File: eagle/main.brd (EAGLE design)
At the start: 100 x 80 mm, 32 parts, among them Q1 BSS97, U1 LTC3789EGNPBF

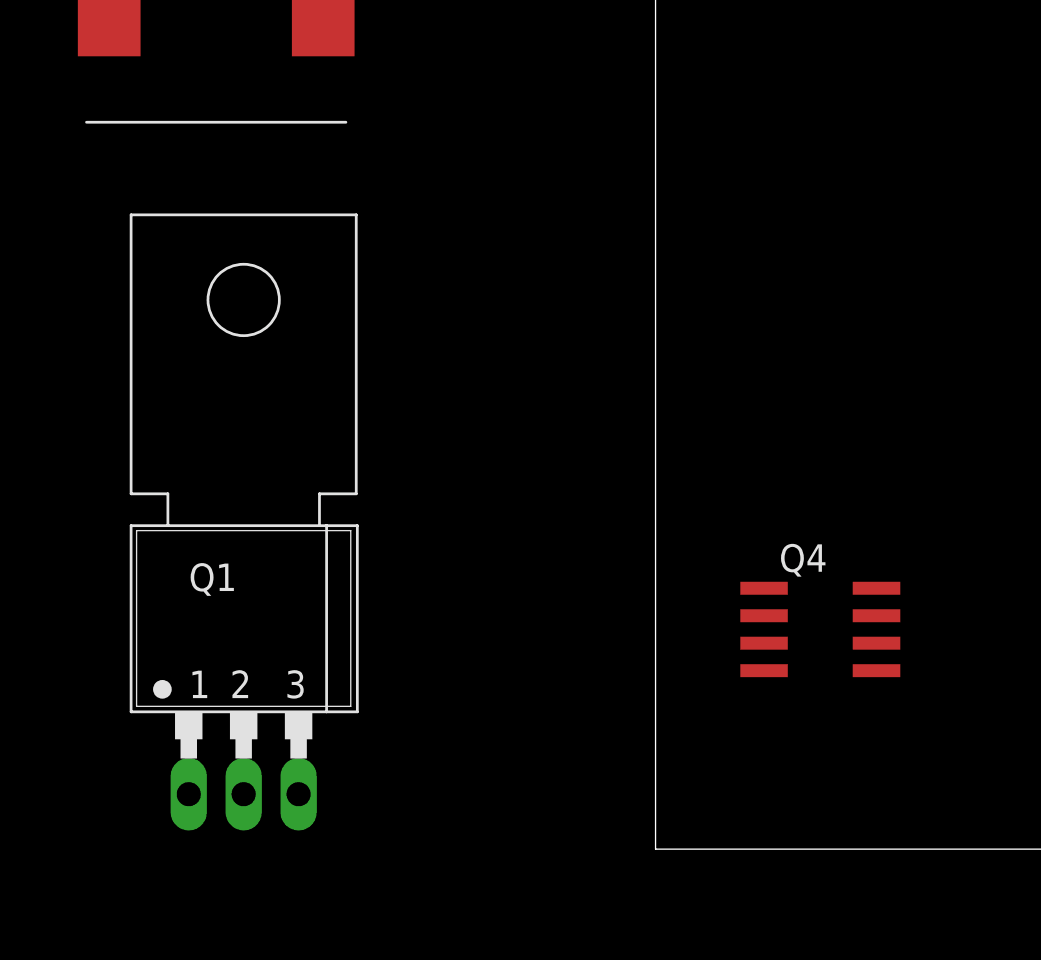
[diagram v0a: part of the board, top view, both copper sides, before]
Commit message: [ update ] sch
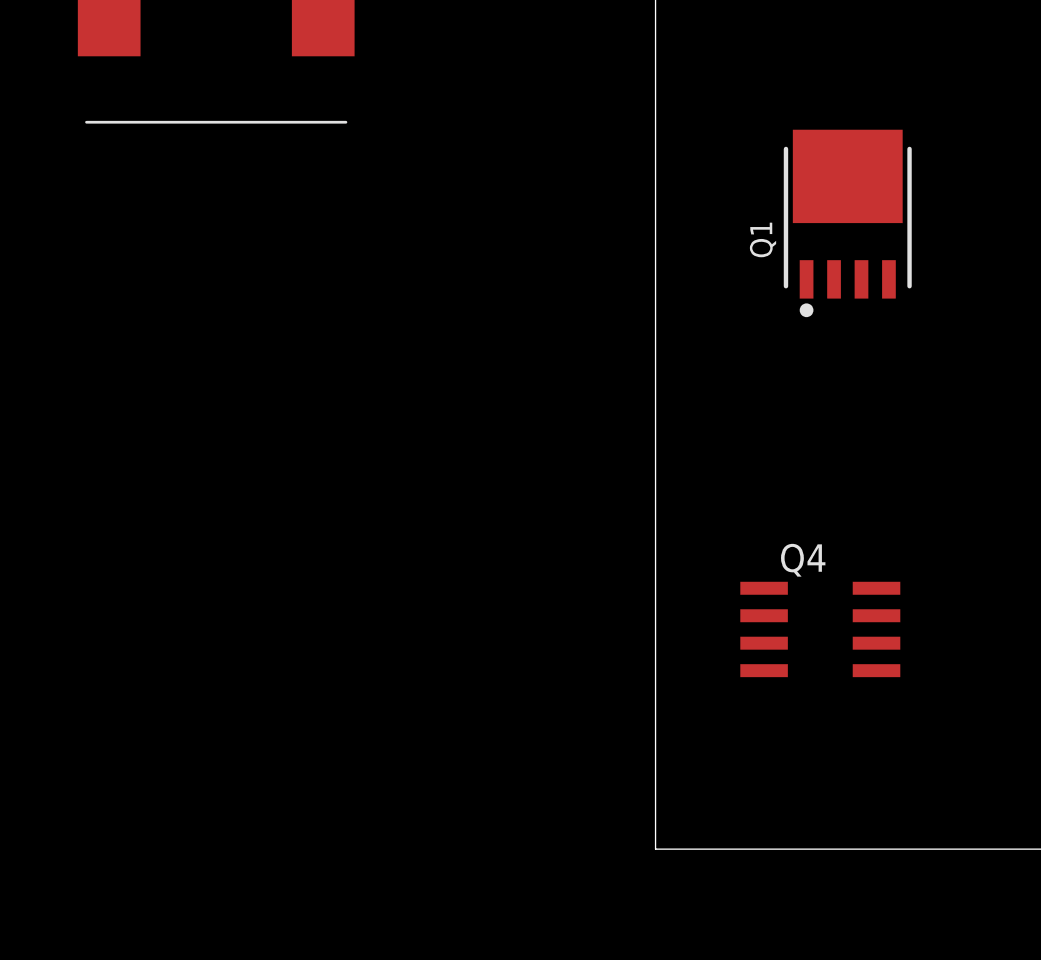
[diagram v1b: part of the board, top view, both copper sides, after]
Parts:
- Q1: value BSS97 -> SQJ886EP; device transistor-fet:TO202 -> transistor-fet:POWERPAK-SO-08
- moved Q1 35.3 mm to (8.89, 29.2)
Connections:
- net SW1: now also Q1.2, Q1.3
- net TG1: now also Q1.4; no longer Q1.3
- net VIN: now also Q1.5-8; no longer Q1.2
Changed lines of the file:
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@@
 <setting verticaltext="up"/>
 </settings>
-<grid distance="0.05" unitdist="inch" unit="inch" style="lines" multiple="1" display="no" altdistance="0.025" altunitdist="inch" altunit="inch"/>
+<grid distance="0.05" unitdist="inch" unit="inch" style="lines" multiple="1" display="yes" altdistance="0.025" altunitdist="inch" altunit="inch"/>
 <layers>
 <layer number="1" name="Top" color="4" fill="1" visible="yes" active="yes"/>
@@
 <element name="C4" library="rcl" package="C1206K" value="1u" x="-35.56" y="71.12"/>
 <element name="C5" library="rcl" package="C1206K" value="4.7u" x="-40.64" y="71.12"/>
-<element name="Q1" library="transistor-fet" package="TO202" value="BSS97" x="-19.05" y="7.62"/>
 <element name="C6" library="rcl" package="C1206K" value="2.2u" x="-45.72" y="71.12"/>
 <element name="C7" library="rcl" package="PANASONIC_A" value="330u" x="-66.04" y="33.02"/>
@@
 <element name="Q3" library="transistor-power" package="SO-08" value="" x="-91.44" y="-21.59"/>
 <element name="Q4" library="transistor-power" package="SO-08" value="" x="7.62" y="10.16" rot="R270"/>
+<element name="Q1" library="transistor-fet" package="POWERPAK-SO-08" value="SQJ886EP" x="8.89" y="29.21"/>
 </elements>
 <signals>
@@
 <contactref element="R10" pad="1"/>
 <contactref element="C8" pad="1"/>
-<contactref element="Q1" pad="2"/>
-<wire x1="-56.032" y1="64.77" x2="-52.3" y2="71.12" width="0" layer="19" extent="1-1"/>
-<wire x1="-51.9938" y1="36.5252" x2="-56.032" y2="64.77" width="0" layer="19" extent="1-1"/>
-<wire x1="-19.05" y1="2.54" x2="-51.9938" y2="36.5252" width="0" layer="19" extent="1-1"/>
+<contactref element="Q1" pad="5-8"/>
+<wire x1="-51.9938" y1="36.5252" x2="8.89" y2="31.115" width="0" layer="19" extent="1-1"/>
+<wire x1="-56.032" y1="64.77" x2="-51.9938" y2="36.5252" width="0" layer="19" extent="1-1"/>
+<wire x1="-52.3" y1="71.12" x2="-56.032" y2="64.77" width="0" layer="19" extent="1-1"/>
 </signal>
 <signal name="SENSE-">
@@
 <signal name="TG1">
 <contactref element="U1" pad="26"/>
-<contactref element="Q1" pad="3"/>
-<wire x1="-47.0662" y1="40.9448" x2="-16.51" y2="2.54" width="0" layer="19" extent="1-1"/>
+<contactref element="Q1" pad="4"/>
+<wire x1="-47.0662" y1="40.9448" x2="10.795" y2="26.3525" width="0" layer="19" extent="1-1"/>
 </signal>
 <signal name="BG2">
@@
 <signal name="SW1">
 <contactref element="U1" pad="27"/>
-<contactref element="Q1" pad="1"/>
 <contactref element="L1" pad="2"/>
 <contactref element="C12" pad="1"/>
@@
 <contactref element="Q2" pad="6"/>
 <contactref element="Q2" pad="7"/>
+<contactref element="Q1" pad="1"/>
+<contactref element="Q1" pad="2"/>
+<contactref element="Q1" pad="3"/>
+<wire x1="8.255" y1="26.3525" x2="6.985" y2="26.3525" width="0" layer="19" extent="1-1"/>
+<wire x1="9.525" y1="26.3525" x2="8.255" y2="26.3525" width="0" layer="19" extent="1-1"/>
+<wire x1="-84.455" y1="-18.99" x2="9.525" y2="26.3525" width="0" layer="19" extent="1-1"/>
 <wire x1="-83.185" y1="-18.99" x2="-84.455" y2="-18.99" width="0" layer="19" extent="1-1"/>
 <wire x1="-81.915" y1="-18.99" x2="-83.185" y2="-18.99" width="0" layer="19" extent="1-1"/>
 <wire x1="-80.645" y1="-18.99" x2="-81.915" y2="-18.99" width="0" layer="19" extent="1-1"/>
 <wire x1="-66.82" y1="-12.7" x2="-80.645" y2="-18.99" width="0" layer="19" extent="1-1"/>
-<wire x1="-21.59" y1="2.54" x2="-66.82" y2="-12.7" width="0" layer="19" extent="1-1"/>
-<wire x1="-15.37" y1="39.37" x2="-21.59" y2="2.54" width="0" layer="19" extent="1-1"/>
-<wire x1="-47.0662" y1="41.6052" x2="-15.37" y2="39.37" width="0" layer="19" extent="1-1"/>
+<wire x1="-47.0662" y1="41.6052" x2="-66.82" y2="-12.7" width="0" layer="19" extent="1-1"/>
 <wire x1="-66.27" y1="64.77" x2="-47.0662" y2="41.6052" width="0" layer="19" extent="1-1"/>
+<wire x1="-15.37" y1="39.37" x2="-47.0662" y2="41.6052" width="0" layer="19" extent="1-1"/>
 </signal>
 <signal name="N$9">
